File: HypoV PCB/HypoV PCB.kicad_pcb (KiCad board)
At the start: 2 copper layers, 59 x 24.5 mm, 13 parts, among them J1 Conn_Header_JST_PH_1x02_P2mm_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

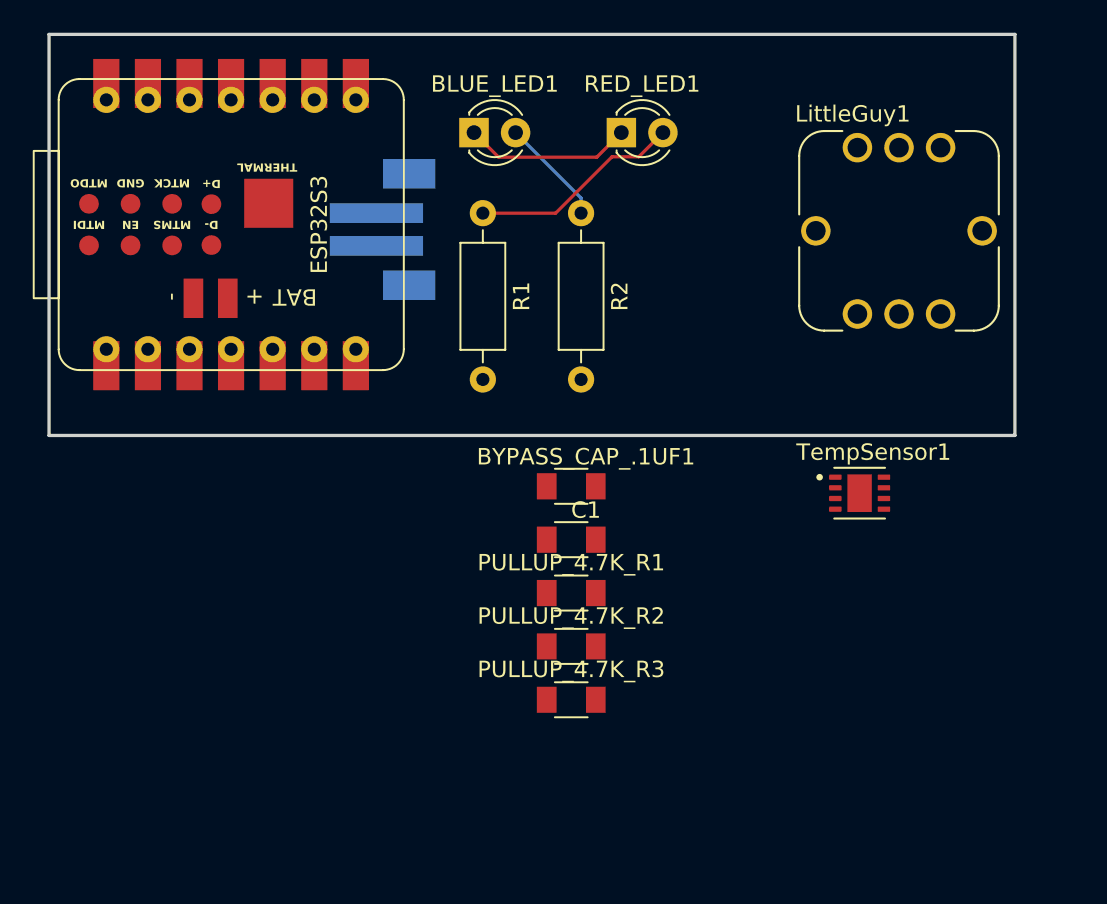
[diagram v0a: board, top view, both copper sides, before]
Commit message: added final pcb stuff
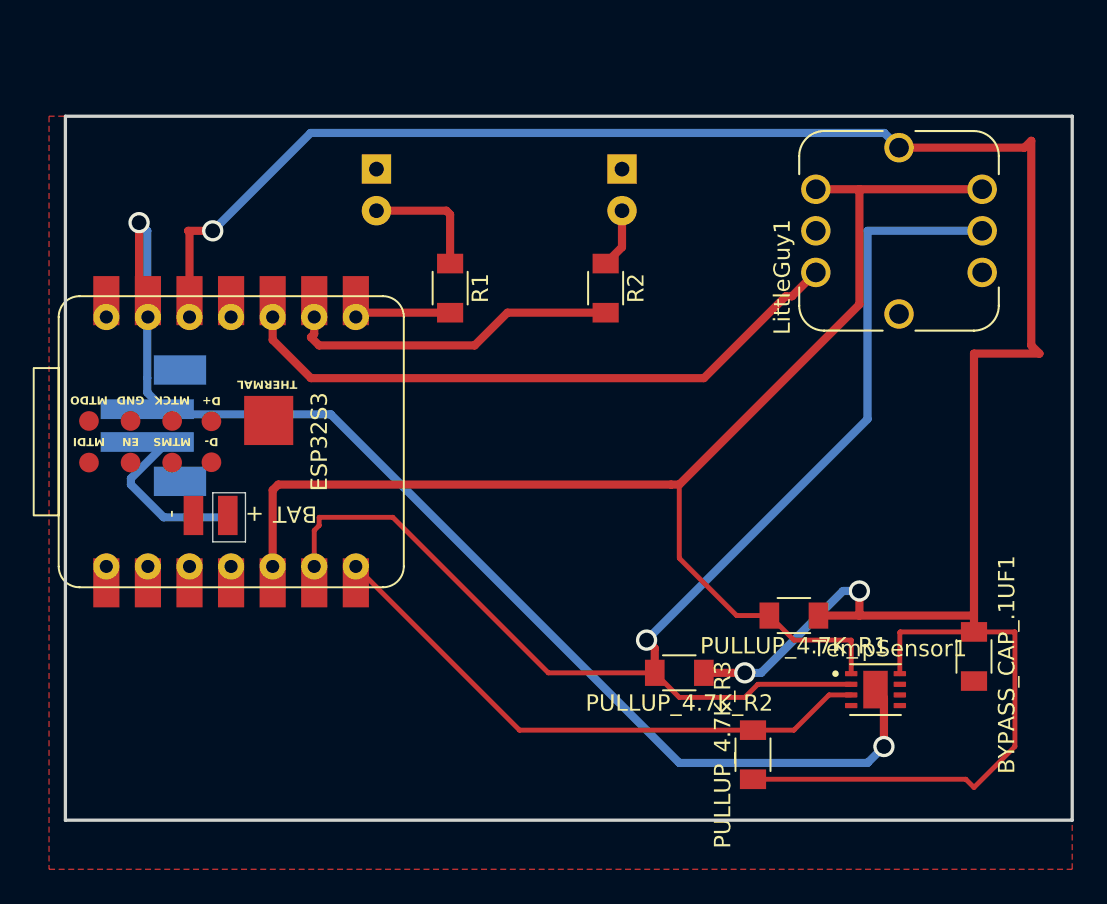
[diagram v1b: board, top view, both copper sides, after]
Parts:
- removed the BYPASS_CAP_.1UF1 at (101.9, 92.6)
- BLUE_LED1, RED_LED1: moved to B.Cu
- R1, R2: footprint Resistor_THT:R_Axial_DIN0207_L6.3mm_D2.5mm_P10.16mm_Horizontal -> PCM_fab:R_1206
- moved BYPASS_CAP_.1UF1 25.6 mm to (126.5, 103.0), turned to -90 degrees
- moved J1 18.4 mm to (76.0, 88.9)
- moved RED_LED1 15.1 mm to (90.0, 73.2), turned to -90 degrees
- moved PULLUP_4.7K_R1 13.7 mm to (115.5, 100.5), turned to 180 degrees
- moved ESP32S3 13.3 mm to (81.1, 89.9)
- moved TempSensor1 12.0 mm to (120.5, 105.0)
- moved PULLUP_4.7K_R3 11.6 mm to (113.0, 109.0), turned to 90 degrees
- moved BLUE_LED1 9.31 mm to (105.0, 73.2), turned to -90 degrees
- moved PULLUP_4.7K_R2 6.79 mm to (108.5, 104.0), turned to 180 degrees
- moved R1 5.00 mm to (94.5, 80.5)
- moved R2 4.82 mm to (104.0, 80.5)
- turned LittleGuy1 to 90 degrees
- renumbered C1 to BYPASS_CAP_.1UF1
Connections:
- ESP32S3 pad 10: unconnected-(ESP32S3-D9-Pad10) -> /D9
- ESP32S3 pad 8: unconnected-(ESP32S3-D7-Pad8) -> Net-(ESP32S3-D7)
- ESP32S3 pad 9: unconnected-(ESP32S3-D8-Pad9) -> Net-(ESP32S3-D8)
- LittleGuy1 pad INT: unconnected-(LittleGuy1-PadINT) -> /D9
- LittleGuy1 pad SDA: unconnected-(LittleGuy1-PadSDA) -> /SDA
- R1 pad 2: unconnected-(R1-Pad2) -> Net-(ESP32S3-D7)
- R2 pad 2: unconnected-(R2-Pad2) -> Net-(ESP32S3-D8)
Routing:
- net +3.3V: track 0.00 -> 150.4 mm, vias 0 -> 3
- net /SDA: track 0.00 -> 81.5 mm
- net /SCL: track 0.00 -> 80.3 mm, vias 0 -> 1
- net GND: track 10.2 -> 73.9 mm, vias 0 -> 2
- net /D9: track 0.00 -> 38.2 mm
- net /OS: track 0.00 -> 35.3 mm
- net Net-(ESP32S3-D8): track 0.00 -> 20.4 mm
- net Net-(ESP32S3-BAT_VIN): track 0.00 -> 10.4 mm
- net Net-(ESP32S3-D7): track 0.00 -> 5.87 mm
- net Net-(RED_LED1-A): track 13.0 -> 7.60 mm
- net Net-(BLUE_LED1-A): track 6.58 -> 3.64 mm
- added copper zone on F.Cu, net GND
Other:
- board size 59 x 24.5 mm -> 61.5 x 43 mm
